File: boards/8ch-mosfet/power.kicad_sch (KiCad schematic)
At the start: 21 parts, among them J3 Screw_Terminal_01x08, J4 Screw_Terminal_01x08, U4 XL1509-5.0

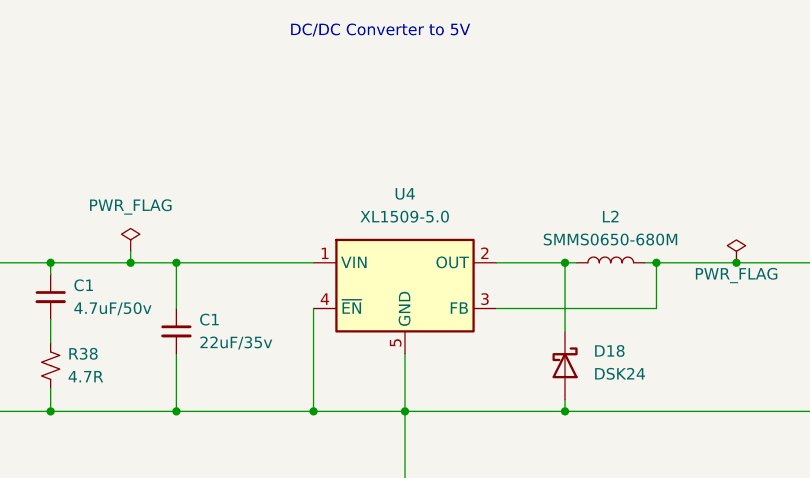
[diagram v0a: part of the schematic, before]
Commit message: reannotated
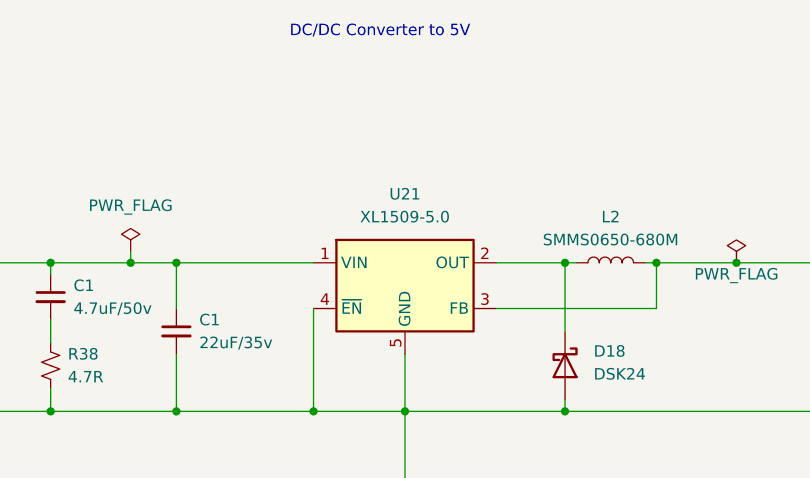
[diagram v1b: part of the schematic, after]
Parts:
- renumbered U4 to U21
